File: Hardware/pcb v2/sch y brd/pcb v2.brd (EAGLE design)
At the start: 80 x 80 mm, 58 parts, among them J1 AVR_SPI_PRG_6PTH, J2 1981584-1, J3 HDMI_OP, J4 JST-3, J5 HDMI_OP, J6 FEMALE 2x3, J7 2X6 FEMALE, Q1 PMBT3904, Q2 PMBT3904, U1 ATMEGA328P, U2 TXS0108EPWR-TSSOP20, U3 ADP3338AKCZ-3.3RL7, U4 DS1307SO8, Y1 CSTCE16M0V53-R0 16MHZ, Y2 MC-306

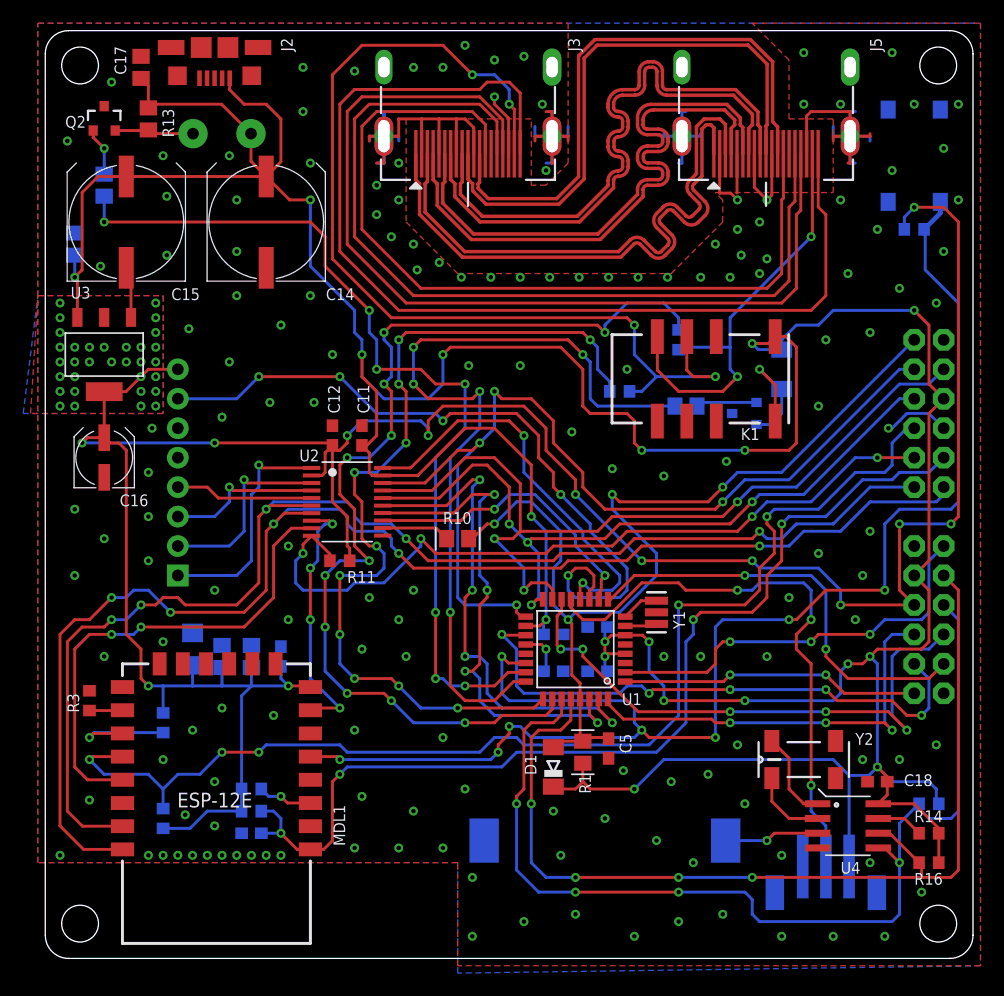
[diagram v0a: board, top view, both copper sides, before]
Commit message: revertir los cambios de osh park
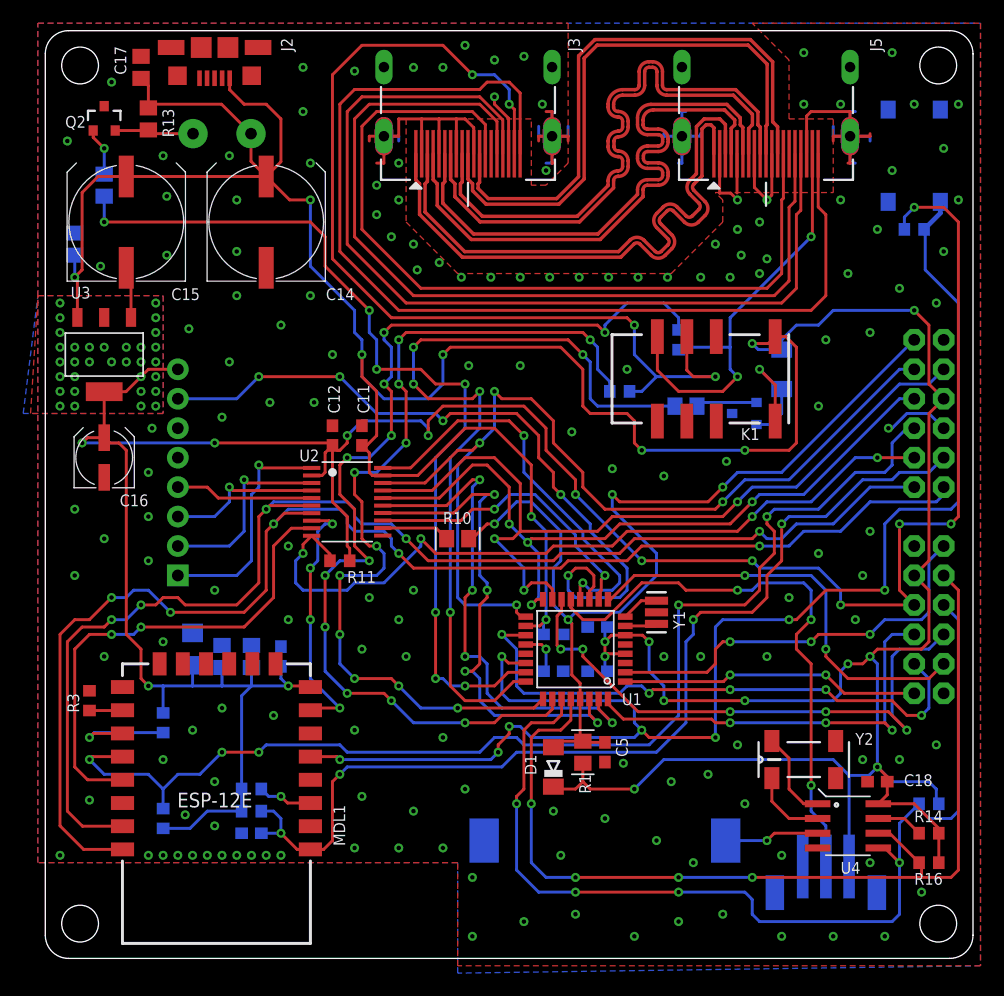
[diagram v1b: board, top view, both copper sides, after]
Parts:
- J3, J5: value HDMI_OP -> HDMI; device partes v2:0471511071_OP -> partes v2:0471511071
- moved C5 0.45 mm to (48.3, 17.8)
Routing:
- net GND: track 121.9 -> 111.7 mm
- net RST_ATM: track 84.8 -> 84.3 mm
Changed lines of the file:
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@@
 <setting verticaltext="up"/>
 </settings>
-<grid distance="0.025" unitdist="inch" unit="inch" style="lines" multiple="1" display="yes" altdistance="0.0125" altunitdist="inch" altunit="inch"/>
+<grid distance="1" unitdist="mm" unit="mm" style="dots" multiple="1" display="yes" altdistance="0.0125" altunitdist="inch" altunit="inch"/>
 <layers>
 <layer number="1" name="Top" color="4" fill="1" visible="yes" active="yes"/>
@@
 </class>
 </classes>
-<designrules name="oshpark-2layer *">
+<designrules name="SeeedStudio_2layer_DRU_no_angle_20140221 *">
 <description language="de">&lt;b&gt;EAGLE Design Rules&lt;/b&gt;
 &lt;p&gt;
@@
 Einstellungen hier und speichern die Design Rules unter
 einem neuen Namen ab.</description>
-<description language="en">&lt;b&gt;Laen's PCB Order Design Rules&lt;/b&gt;
+<description language="en">&lt;b&gt;EAGLE Design Rules&lt;/b&gt;
 &lt;p&gt;
-Please make sure your boards conform to these design rules.</description>
+The default Design Rules have been set to cover
+a wide range of applications. Your particular design
+may have different requirements, so please make the
+necessary adjustments and save your customized
+design rules under a new name.</description>
+<description language="zh">&lt;b&gt;Seeed Studio EAGLE Design Rules&lt;/b&gt;
+</description>
 <param name="layerSetup" value="(1*16)"/>
-<param name="mtCopper" value="0.0356mm 0.0356mm 0.0356mm 0.0356mm 0.0356mm 0.0356mm 0.0356mm 0.0356mm 0.0356mm 0.0356mm 0.0356mm 0.0356mm 0.0356mm 0.0356mm 0.0356mm 0.0356mm"/>
-<param name="mtIsolate" value="1.5011mm 0.1499mm 0.2007mm 0.1499mm 0.2007mm 0.1499mm 0.2007mm 0.1499mm 0.2007mm 0.1499mm 0.2007mm 0.1499mm 0.2007mm 0.1499mm 0.2007mm"/>
+<param name="mtCopper" value="0.035mm 0.0175mm 0.035mm 0.035mm 0.035mm 0.035mm 0.035mm 0.035mm 0.035mm 0.035mm 0.035mm 0.035mm 0.035mm 0.035mm 0.0175mm 0.035mm"/>
+<param name="mtIsolate" value="1.5mm 1.1mm 0.2mm 0.15mm 0.2mm 0.15mm 0.2mm 0.15mm 0.2mm 0.15mm 0.2mm 0.15mm 0.2mm 0.15mm 0.2mm"/>
 <param name="mdWireWire" value="6mil"/>
 <param name="mdWirePad" value="6mil"/>
@@
 <param name="mdPadVia" value="6mil"/>
 <param name="mdViaVia" value="6mil"/>
-<param name="mdSmdPad" value="6mil"/>
-<param name="mdSmdVia" value="6mil"/>
-<param name="mdSmdSmd" value="6mil"/>
+<param name="mdSmdPad" value="0mil"/>
+<param name="mdSmdVia" value="0mil"/>
+<param name="mdSmdSmd" value="0mil"/>
 <param name="mdViaViaSameLayer" value="8mil"/>
 <param name="mnLayersViaInSmd" value="2"/>
-<param name="mdCopperDimension" value="15mil"/>
-<param name="mdDrill" value="6mil"/>
+<param name="mdCopperDimension" value="16mil"/>
+<param name="mdDrill" value="10mil"/>
 <param name="mdSmdStop" value="0mil"/>
 <param name="msWidth" value="6mil"/>
-<param name="msDrill" value="13mil"/>
-<param name="msMicroVia" value="13mil"/>
+<param name="msDrill" value="12mil"/>
+<param name="msMicroVia" value="12mil"/>
 <param name="msBlindViaRatio" value="0.5"/>
 <param name="rvPadTop" value="0.25"/>
@@
 <param name="rvMicroViaOuter" value="0.25"/>
 <param name="rvMicroViaInner" value="0.25"/>
-<param name="rlMinPadTop" value="7mil"/>
+<param name="rlMinPadTop" value="10mil"/>
 <param name="rlMaxPadTop" value="20mil"/>
-<param name="rlMinPadInner" value="7mil"/>
+<param name="rlMinPadInner" value="10mil"/>
 <param name="rlMaxPadInner" value="20mil"/>
-<param name="rlMinPadBottom" value="7mil"/>
+<param name="rlMinPadBottom" value="10mil"/>
 <param name="rlMaxPadBottom" value="20mil"/>
-<param name="rlMinViaOuter" value="7mil"/>
+<param name="rlMinViaOuter" value="6mil"/>
 <param name="rlMaxViaOuter" value="20mil"/>
-<param name="rlMinViaInner" value="7mil"/>
+<param name="rlMinViaInner" value="6mil"/>
 <param name="rlMaxViaInner" value="20mil"/>
 <param name="rlMinMicroViaOuter" value="4mil"/>
@@
 <param name="psTop" value="-1"/>
 <param name="psBottom" value="-1"/>
-<param name="psFirst" value="-1"/>
+<param name="psFirst" value="0"/>
 <param name="psElongationLong" value="100"/>
 <param name="psElongationOffset" value="100"/>
 <param name="mvStopFrame" value="1"/>
 <param name="mvCreamFrame" value="0"/>
-<param name="mlMinStopFrame" value="2.5mil"/>
-<param name="mlMaxStopFrame" value="2.5mil"/>
+<param name="mlMinStopFrame" value="2mil"/>
+<param name="mlMaxStopFrame" value="2mil"/>
 <param name="mlMinCreamFrame" value="0mil"/>
 <param name="mlMaxCreamFrame" value="0mil"/>
-<param name="mlViaStopLimit" value="0mil"/>
+<param name="mlViaStopLimit" value="100mil"/>
 <param name="srRoundness" value="0"/>
 <param name="srMinRoundness" value="0mil"/>
@@
 <param name="dpGapFactor" value="2.5"/>
 <param name="checkGrid" value="0"/>
-<param name="checkAngle" value="0"/>
+<param name="checkAngle" value="1"/>
 <param name="checkFont" value="1"/>
-<param name="checkRestrict" value="1"/>
+<param name="checkRestrict" value="0"/>
 <param name="useDiameter" value="13"/>
 <param name="maxErrors" value="50"/>
@@
 <attribute name="VALUE" x="46.228" y="14.859" size="1.016" layer="27" ratio="16" rot="R90"/>
 </element>
-<element name="C5" library="rcl" package="C0603" value="100nF" x="48.5775" y="18.0975" smashed="yes" rot="R270">
-<attribute name="NAME" x="49.53" y="19.3675" size="1.016" layer="25" ratio="16" rot="R270"/>
-<attribute name="VALUE" x="46.6725" y="18.7325" size="1.016" layer="27" ratio="16" rot="R270"/>
+<element name="C5" library="rcl" package="C0603" value="100nF" x="48.26" y="17.78" smashed="yes" rot="R270">
+<attribute name="NAME" x="49.2125" y="19.05" size="1.016" layer="25" ratio="16" rot="R270"/>
+<attribute name="VALUE" x="46.355" y="18.415" size="1.016" layer="27" ratio="16" rot="R270"/>
 </element>
 <element name="C2" library="rcl" package="C0603" value="100nF" x="47.625" y="24.765" smashed="yes" rot="MR0">
@@
 <attribute name="VALUE" x="65.913" y="52.451" size="1.016" layer="28" ratio="16" rot="MR270"/>
 </element>
-<element name="J5" library="partes v2" package="0471511071_OP" value="HDMI_OP" x="62.15" y="73.14" locked="yes" smashed="yes" rot="R180">
+<element name="J5" library="partes v2" package="0471511071" value="HDMI" x="62.15" y="73.14" locked="yes" smashed="yes" rot="R180">
 <attribute name="NAME" x="71.12" y="79.375" size="1.016" layer="25" font="vector" ratio="16" rot="R270"/>
 </element>
-<element name="J3" library="partes v2" package="0471511071_OP" value="HDMI_OP" x="36.45" y="73.14" locked="yes" smashed="yes" rot="R180">
+<element name="J3" library="partes v2" package="0471511071" value="HDMI" x="36.45" y="73.14" locked="yes" smashed="yes" rot="R180">
 <attribute name="NAME" x="45.085" y="79.375" size="1.016" layer="25" ratio="16" rot="R270"/>
 </element>
@@
 <wire x1="69.4" y1="68.58" x2="69.215" y2="68.58" width="0.254" layer="1"/>
 <wire x1="67.945" y1="70.9" x2="67.945" y2="70.485" width="0.254" layer="1"/>
+<wire x1="29.2" y1="70.9" x2="30.48" y2="70.9" width="0.254" layer="16"/>
+<wire x1="30.48" y1="70.9" x2="30.48" y2="70.485" width="0.254" layer="16"/>
 <wire x1="27.94" y1="70.9" x2="30.48" y2="70.9" width="0.254" layer="1"/>
 <wire x1="30.48" y1="70.9" x2="30.48" y2="72.39" width="0.254" layer="1"/>
-<wire x1="42.2275" y1="70.9" x2="42.2275" y2="71.755" width="0.254" layer="16"/>
-<wire x1="42.2275" y1="70.9" x2="45.085" y2="70.9" width="0.254" layer="16"/>
+<wire x1="42.545" y1="70.9" x2="42.545" y2="71.755" width="0.254" layer="16"/>
+<wire x1="42.545" y1="70.9" x2="45.085" y2="70.9" width="0.254" layer="16"/>
 <wire x1="45.085" y1="70.9" x2="45.085" y2="71.755" width="0.254" layer="16"/>
-<wire x1="42.2275" y1="70.9" x2="42.2275" y2="70.485" width="0.254" layer="1"/>
-<wire x1="42.2275" y1="70.9" x2="43.7" y2="70.9" width="0.254" layer="1"/>
+<wire x1="42.545" y1="70.9" x2="42.545" y2="70.485" width="0.254" layer="1"/>
+<wire x1="42.545" y1="70.9" x2="43.7" y2="70.9" width="0.254" layer="1"/>
 <wire x1="43.7" y1="70.9" x2="45.085" y2="70.9" width="0.254" layer="1"/>
 <wire x1="45.085" y1="70.9" x2="45.085" y2="70.485" width="0.254" layer="1"/>
@@
 <via x="56.515" y="26.035" extent="1-16" drill="0.381" diameter="0.7874"/>
 <via x="59.69" y="18.415" extent="1-16" drill="0.381" diameter="0.7874"/>
-<via x="49.8475" y="16.1925" extent="1-16" drill="0.381" diameter="0.7874"/>
+<via x="49.8475" y="16.8275" extent="1-16" drill="0.381" diameter="0.7874"/>
 <via x="53.975" y="15.24" extent="1-16" drill="0.381" diameter="0.7874"/>
 <via x="57.15" y="15.875" extent="1-16" drill="0.381" diameter="0.7874"/>
@@
 <wire x1="74.295" y1="46.99" x2="76.2" y2="46.99" width="0.254" layer="16"/>
 <wire x1="76.2" y1="46.99" x2="77.47" y2="45.72" width="0.254" layer="16"/>
-<wire x1="29.2" y1="70.9" x2="27.94" y2="70.9" width="0.254" layer="16"/>
-<wire x1="27.94" y1="70.9" x2="27.94" y2="70.485" width="0.254" layer="16"/>
-<wire x1="30.48" y1="70.9" x2="30.48" y2="70.485" width="0.254" layer="16"/>
-<wire x1="29.2" y1="70.9" x2="29.2" y2="73.025" width="0.254" layer="16"/>
-<wire x1="29.2" y1="73.025" x2="29.21" y2="73.025" width="0.254" layer="16"/>
-<wire x1="29.845" y1="73.025" x2="29.21" y2="73.025" width="0.254" layer="16"/>
-<wire x1="29.21" y1="73.025" x2="29.21" y2="68.58" width="0.254" layer="16"/>
-<wire x1="29.21" y1="68.58" x2="28.575" y2="68.58" width="0.254" layer="16"/>
-<wire x1="30.48" y1="70.9" x2="29.2" y2="70.9" width="0.254" layer="16"/>
 </signal>
 <signal name="+5V">
@@
 <contactref element="R10" pad="2"/>
 <wire x1="46.355" y1="18.73" x2="46.455" y2="18.63" width="0.254" layer="1"/>
-<wire x1="46.455" y1="18.63" x2="46.99" y2="19.05" width="0.254" layer="1"/>
-<wire x1="46.99" y1="19.05" x2="48.475" y2="19.05" width="0.254" layer="1"/>
-<wire x1="48.475" y1="19.05" x2="48.5775" y2="18.9475" width="0.254" layer="1"/>
+<wire x1="46.455" y1="18.63" x2="48.26" y2="18.63" width="0.254" layer="1"/>
 <wire x1="46.355" y1="18.73" x2="46.12" y2="18.965" width="0.254" layer="1"/>
 <wire x1="46.12" y1="18.965" x2="46.12" y2="22.3774" width="0.254" layer="1"/>
